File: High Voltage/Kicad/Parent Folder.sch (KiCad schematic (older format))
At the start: 25 parts

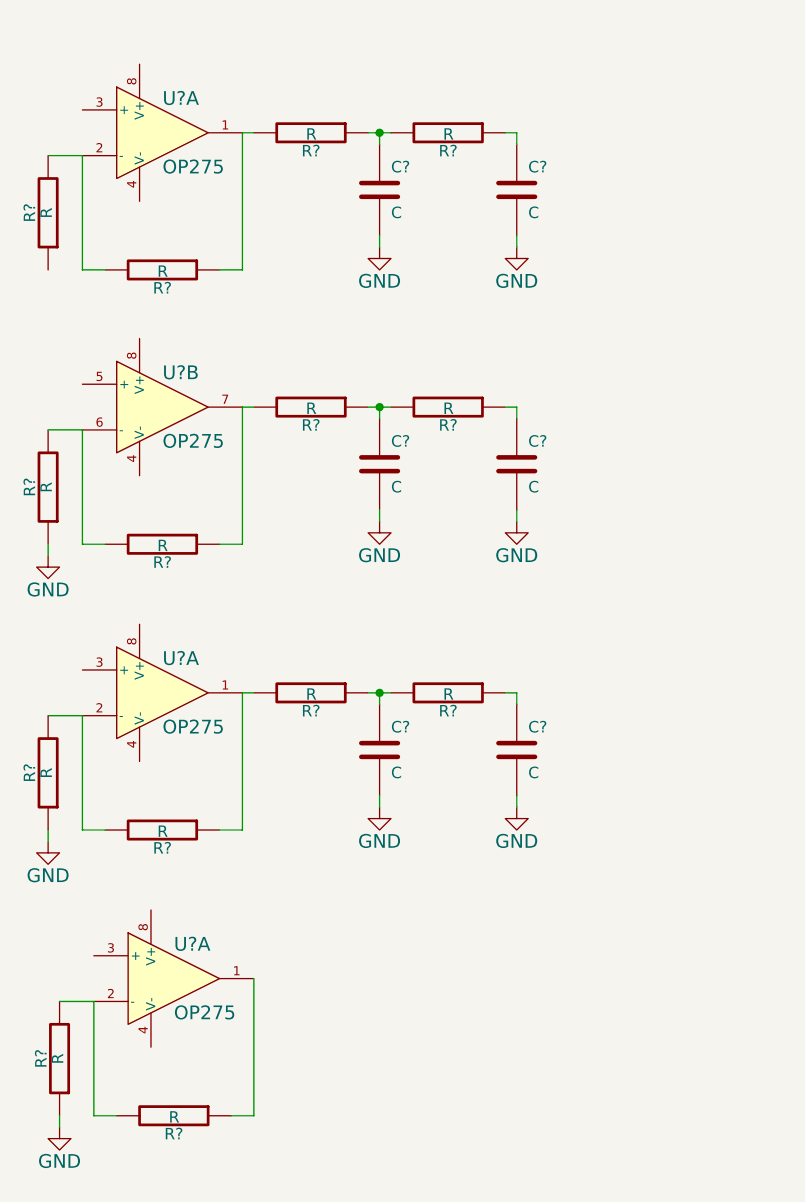
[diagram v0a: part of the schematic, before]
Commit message: Loading characterization & other comments
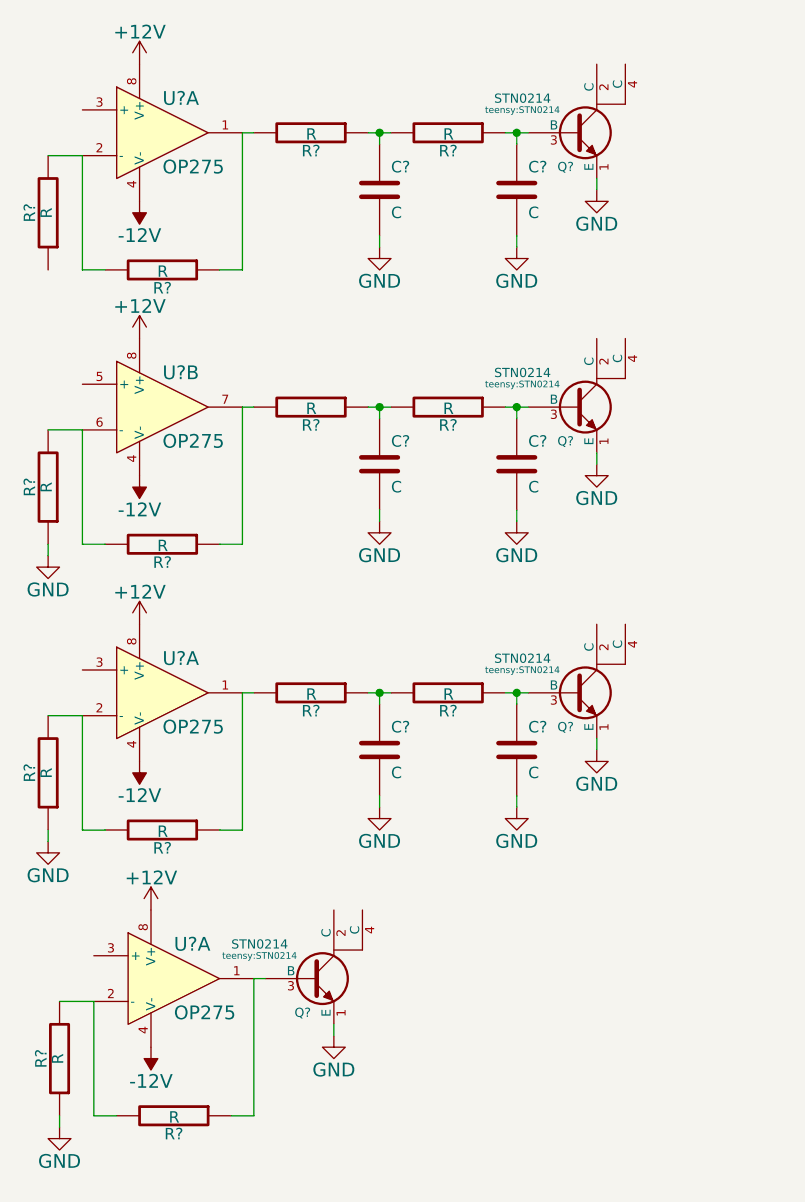
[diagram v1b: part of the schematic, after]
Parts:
- added Q? (x4): STN0214, teensy:STN0214, symbol STN0214
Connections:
- net GND: now also Q?.1 (E), Q?.1 (E), Q?.1 (E), Q?.1 (E)
- net -12V: now reaches U?.4 (V-)
- net -12V: now also U?.4 (V-), U?.4 (V-), U?.4 (V-)
- net +12V: now reaches U?.8 (V+)
- net +12V: now also U?.8 (V+), U?.8 (V+), U?.8 (V+)
- net at C?.1, R?.1: now also Q?.3 (B) (x3)
- net at R?.1, U?.1: now also Q?.3 (B)
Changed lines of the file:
@@
 	1    0    0    -1
 $EndComp
-Wire Wire Line
-	2900 1500 3000 1500
-Wire Wire Line
-	2950 1550 2950 1500
-Connection ~ 2950 1500
-Wire Wire Line
-	2900 2700 3000 2700
-Wire Wire Line
-	2950 2750 2950 2700
-Connection ~ 2950 2700
-Wire Wire Line
-	2900 3950 3000 3950
-Wire Wire Line
-	2950 4000 2950 3950
-Connection ~ 2950 3950
 $Comp
 L GND #PWR?
@@
 	1    0    0    -1
 $EndComp
-Wire Wire Line
-	2950 1950 2950 2000
-Wire Wire Line
-	2950 4400 2950 4450
-Wire Wire Line
-	2950 3150 2950 3200
 $Comp
 L C C?
@@
 	1    0    0    -1
 $EndComp
-Wire Wire Line
-	3550 3150 3550 3200
 $Comp
 L C C?
@@
 	1    0    0    -1
 $EndComp
-Wire Wire Line
-	3550 1950 3550 2000
 $Comp
 L C C?
@@
 	1    0    0    -1
 $EndComp
-Wire Wire Line
-	3550 4400 3550 4450
-Wire Wire Line
-	3500 1500 3550 1500
-Wire Wire Line
-	3550 1500 3550 1550
-Wire Wire Line
-	3500 2700 3550 2700
-Wire Wire Line
-	3550 2700 3550 2750
-Wire Wire Line
-	3500 3950 3550 3950
-Wire Wire Line
-	3550 3950 3550 4000
 $Comp
 L R R?
@@
 	0    1    1    0
 $EndComp
-Wire Wire Line
-	1650 1600 1650 2100
-Wire Wire Line
-	1650 2100 1750 2100
-Wire Wire Line
-	2250 2100 2350 2100
-Wire Wire Line
-	2350 2100 2350 1500
 $Comp
 L R R?
@@
 	-1   0    0    1
 $EndComp
-Wire Wire Line
-	1500 1600 1650 1600
 $Comp
 L R R?
@@
 	0    1    1    0
 $EndComp
-Wire Wire Line
-	1650 2800 1650 3300
-Wire Wire Line
-	1650 3300 1750 3300
-Wire Wire Line
-	2250 3300 2350 3300
-Wire Wire Line
-	2350 3300 2350 2700
 $Comp
 L R R?
@@
 	-1   0    0    1
 $EndComp
-Wire Wire Line
-	1500 2800 1650 2800
 $Comp
 L OP275 U?
@@
 	0    1    1    0
 $EndComp
-Wire Wire Line
-	1650 4050 1650 4550
-Wire Wire Line
-	1650 4550 1750 4550
-Wire Wire Line
-	2250 4550 2350 4550
-Wire Wire Line
-	2350 4550 2350 3950
 $Comp
 L R R?
@@
 	-1   0    0    1
 $EndComp
-Wire Wire Line
-	1500 4050 1650 4050
 $Comp
 L OP275 U?
@@
 	0    1    1    0
 $EndComp
-Wire Wire Line
-	1700 5300 1700 5800
-Wire Wire Line
-	1700 5800 1800 5800
-Wire Wire Line
-	2300 5800 2400 5800
-Wire Wire Line
-	2400 5800 2400 5200
 $Comp
 L R R?
@@
 	-1   0    0    1
 $EndComp
-Wire Wire Line
-	1550 5300 1700 5300
-Wire Wire Line
-	2350 1500 2400 1500
-Wire Wire Line
-	2350 2700 2400 2700
-Wire Wire Line
-	2350 3950 2400 3950
 $Comp
 L GND #PWR?
@@
 	1    0    0    -1
 $EndComp
-Wire Wire Line
-	1500 3300 1500 3350
-Wire Wire Line
-	1500 4550 1500 4600
 $Comp
 L GND #PWR?
@@
 	1    0    0    -1
 $EndComp
+$Comp
+L STN0214 Q?
+U 1 1 54F334D3
+P 3800 1500
+F 0 "Q?" H 3800 1351 40  0000 R CNN
+F 1 "STN0214" H 3700 1650 40  0000 R CNN
+F 2 "teensy:STN0214" H 3575 1600 29  0000 C CNN
+F 3 "" H 3800 1500 60  0000 C CNN
+	1    3800 1500
+	1    0    0    -1
+$EndComp
+$Comp
+L STN0214 Q?
+U 1 1 54F3354C
+P 3800 2700
+F 0 "Q?" H 3800 2551 40  0000 R CNN
+F 1 "STN0214" H 3700 2850 40  0000 R CNN
+F 2 "teensy:STN0214" H 3575 2800 29  0000 C CNN
+F 3 "" H 3800 2700 60  0000 C CNN
+	1    3800 2700
+	1    0    0    -1
+$EndComp
+$Comp
+L STN0214 Q?
+U 1 1 54F33607
+P 3800 3950
+F 0 "Q?" H 3800 3801 40  0000 R CNN
+F 1 "STN0214" H 3700 4100 40  0000 R CNN
+F 2 "teensy:STN0214" H 3575 4050 29  0000 C CNN
+F 3 "" H 3800 3950 60  0000 C CNN
+	1    3800 3950
+	1    0    0    -1
+$EndComp
+$Comp
+L STN0214 Q?
+U 1 1 54F336C8
+P 2650 5200
+F 0 "Q?" H 2650 5051 40  0000 R CNN
+F 1 "STN0214" H 2550 5350 40  0000 R CNN
+F 2 "teensy:STN0214" H 2425 5300 29  0000 C CNN
+F 3 "" H 2650 5200 60  0000 C CNN
+	1    2650 5200
+	1    0    0    -1
+$EndComp
+$Comp
+L GND #PWR?
+U 1 1 54F33797
+P 3900 4200
+F 0 "#PWR?" H 3900 3950 60  0001 C CNN
+F 1 "GND" H 3900 4050 60  0000 C CNN
+F 2 "" H 3900 4200 60  0000 C CNN
+F 3 "" H 3900 4200 60  0000 C CNN
+	1    3900 4200
+	1    0    0    -1
+$EndComp
+$Comp
+L GND #PWR?
+U 1 1 54F3381F
+P 3900 2950
+F 0 "#PWR?" H 3900 2700 60  0001 C CNN
+F 1 "GND" H 3900 2800 60  0000 C CNN
+F 2 "" H 3900 2950 60  0000 C CNN
+F 3 "" H 3900 2950 60  0000 C CNN
+	1    3900 2950
+	1    0    0    -1
+$EndComp
+$Comp
+L GND #PWR?
+U 1 1 54F338E1
+P 3900 1750
+F 0 "#PWR?" H 3900 1500 60  0001 C CNN
+F 1 "GND" H 3900 1600 60  0000 C CNN
+F 2 "" H 3900 1750 60  0000 C CNN
+F 3 "" H 3900 1750 60  0000 C CNN
+	1    3900 1750
+	1    0    0    -1
+$EndComp
+$Comp
+L GND #PWR?
+U 1 1 54F33A34
+P 2750 5450
+F 0 "#PWR?" H 2750 5200 60  0001 C CNN
+F 1 "GND" H 2750 5300 60  0000 C CNN
+F 2 "" H 2750 5450 60  0000 C CNN
+F 3 "" H 2750 5450 60  0000 C CNN
+	1    2750 5450
+	1    0    0    -1
+$EndComp
+Wire Wire Line
+	2900 1500 3000 1500
+Wire Wire Line
+	2950 1550 2950 1500
+Connection ~ 2950 1500
+Wire Wire Line
+	2900 2700 3000 2700
+Wire Wire Line
+	2950 2750 2950 2700
+Connection ~ 2950 2700
+Wire Wire Line
+	2900 3950 3000 3950
+Wire Wire Line
+	2950 4000 2950 3950
+Connection ~ 2950 3950
+Wire Wire Line
+	2950 1950 2950 2000
+Wire Wire Line
+	2950 4400 2950 4450
+Wire Wire Line
+	2950 3150 2950 3200
+Wire Wire Line
+	3550 3150 3550 3200
+Wire Wire Line
+	3550 1950 3550 2000
+Wire Wire Line
+	3550 4400 3550 4450
+Wire Wire Line
+	3500 1500 3600 1500
+Wire Wire Line
+	3550 1500 3550 1550
+Wire Wire Line
+	3500 2700 3600 2700
+Wire Wire Line
+	3550 2700 3550 2750
+Wire Wire Line
+	3500 3950 3600 3950
+Wire Wire Line
+	3550 3950 3550 4000
+Wire Wire Line
+	1650 1600 1650 2100
+Wire Wire Line
+	1650 2100 1750 2100
+Wire Wire Line
+	2250 2100 2350 2100
+Wire Wire Line
+	2350 2100 2350 1500
+Wire Wire Line
+	1500 1600 1650 1600
+Wire Wire Line
+	1650 2800 1650 3300
+Wire Wire Line
+	1650 3300 1750 3300
+Wire Wire Line
+	2250 3300 2350 3300
+Wire Wire Line
+	2350 3300 2350 2700
+Wire Wire Line
+	1500 2800 1650 2800
+Wire Wire Line
+	1650 4050 1650 4550
+Wire Wire Line
+	1650 4550 1750 4550
+Wire Wire Line
+	2250 4550 2350 4550
+Wire Wire Line
+	2350 4550 2350 3950
+Wire Wire Line
+	1500 4050 1650 4050
+Wire Wire Line
+	1700 5300 1700 5800
+Wire Wire Line
+	1700 5800 1800 5800
+Wire Wire Line
+	2300 5800 2400 5800
+Wire Wire Line
+	2400 5800 2400 5200
+Wire Wire Line
+	1550 5300 1700 5300
+Wire Wire Line
+	2350 1500 2400 1500
+Wire Wire Line
+	2350 2700 2400 2700
+Wire Wire Line
+	2350 3950 2400 3950
+Wire Wire Line
+	1500 3300 1500 3350
+Wire Wire Line
+	1500 4550 1500 4600
 Wire Wire Line
 	1550 5850 1550 5800
+Wire Wire Line
+	2750 5400 2750 5450
+Wire Wire Line
+	3900 4200 3900 4150
+Wire Wire Line
+	2400 5200 2450 5200
+Connection ~ 3550 3950
+Connection ~ 3550 2700
+Wire Wire Line
+	3900 2900 3900 2950
+Wire Wire Line
+	3900 1700 3900 1750
+Connection ~ 3550 1500
+$Comp
+L +12V #PWR?
+U 1 1 54F4C6A5
+P 1950 4900
+F 0 "#PWR?" H 1950 4750 60  0001 C CNN
+F 1 "+12V" H 1950 5040 60  0000 C CNN
+F 2 "" H 1950 4900 60  0000 C CNN
+F 3 "" H 1950 4900 60  0000 C CNN
+	1    1950 4900
+	1    0    0    -1
+$EndComp
+$Comp
+L +12V #PWR?
+U 1 1 54F4CCF4
+P 1900 3650
+F 0 "#PWR?" H 1900 3500 60  0001 C CNN
+F 1 "+12V" H 1900 3790 60  0000 C CNN
+F 2 "" H 1900 3650 60  0000 C CNN
+F 3 "" H 1900 3650 60  0000 C CNN
+	1    1900 3650
+	1    0    0    -1
+$EndComp
+$Comp
+L +12V #PWR?
+U 1 1 54F4CD08
+P 1900 2400
+F 0 "#PWR?" H 1900 2250 60  0001 C CNN
+F 1 "+12V" H 1900 2540 60  0000 C CNN
+F 2 "" H 1900 2400 60  0000 C CNN
+F 3 "" H 1900 2400 60  0000 C CNN
+	1    1900 2400
+	1    0    0    -1
+$EndComp
+$Comp
+L +12V #PWR?
+U 1 1 54F4CD56
+P 1900 1200
+F 0 "#PWR?" H 1900 1050 60  0001 C CNN
+F 1 "+12V" H 1900 1340 60  0000 C CNN
+F 2 "" H 1900 1200 60  0000 C CNN
+F 3 "" H 1900 1200 60  0000 C CNN
+	1    1900 1200
+	1    0    0    -1
+$EndComp
+$Comp
+L -12V #PWR?
+U 1 1 54F4CDA4
+P 1900 1800
+F 0 "#PWR?" H 1900 1900 20  0001 C CNN
+F 1 "-12V" H 1900 1950 60  0000 C CNN
+F 2 "" H 1900 1800 60  0000 C CNN
+F 3 "" H 1900 1800 60  0000 C CNN
+	1    1900 1800
+	-1   0    0    1
+$EndComp
+$Comp
+L -12V #PWR?
+U 1 1 54F4CE58
+P 1900 3000
+F 0 "#PWR?" H 1900 3100 20  0001 C CNN
+F 1 "-12V" H 1900 3150 60  0000 C CNN
+F 2 "" H 1900 3000 60  0000 C CNN
+F 3 "" H 1900 3000 60  0000 C CNN
+	1    1900 3000
+	-1   0    0    1
+$EndComp
+$Comp
+L -12V #PWR?
+U 1 1 54F4CEE0
+P 1900 4250
+F 0 "#PWR?" H 1900 4350 20  0001 C CNN
+F 1 "-12V" H 1900 4400 60  0000 C CNN
+F 2 "" H 1900 4250 60  0000 C CNN
+F 3 "" H 1900 4250 60  0000 C CNN
+	1    1900 4250
+	-1   0    0    1
+$EndComp
+$Comp
+L -12V #PWR?
+U 1 1 54F4CF68
+P 1950 5500
+F 0 "#PWR?" H 1950 5600 20  0001 C CNN
+F 1 "-12V" H 1950 5650 60  0000 C CNN
+F 2 "" H 1950 5500 60  0000 C CNN
+F 3 "" H 1950 5500 60  0000 C CNN
+	1    1950 5500
+	-1   0    0    1
+$EndComp
 $EndSCHEMATC
